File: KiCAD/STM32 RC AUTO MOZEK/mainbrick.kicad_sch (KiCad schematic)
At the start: 29 parts, among them J8 Conn_01x03_Socket, U10 ACS712xLCTR-20A, U11 ACS712xLCTR-20A, U13 STM32F030C8Tx, U2 SHT4x, U4 ACS712xLCTR-20A, U5 NRF24L01_Breakout, U7 ACS712xLCTR-20A, U8 ACS712xLCTR-20A, U9 ACS712xLCTR-20A, Y1 Crystal, Y2 Crystal

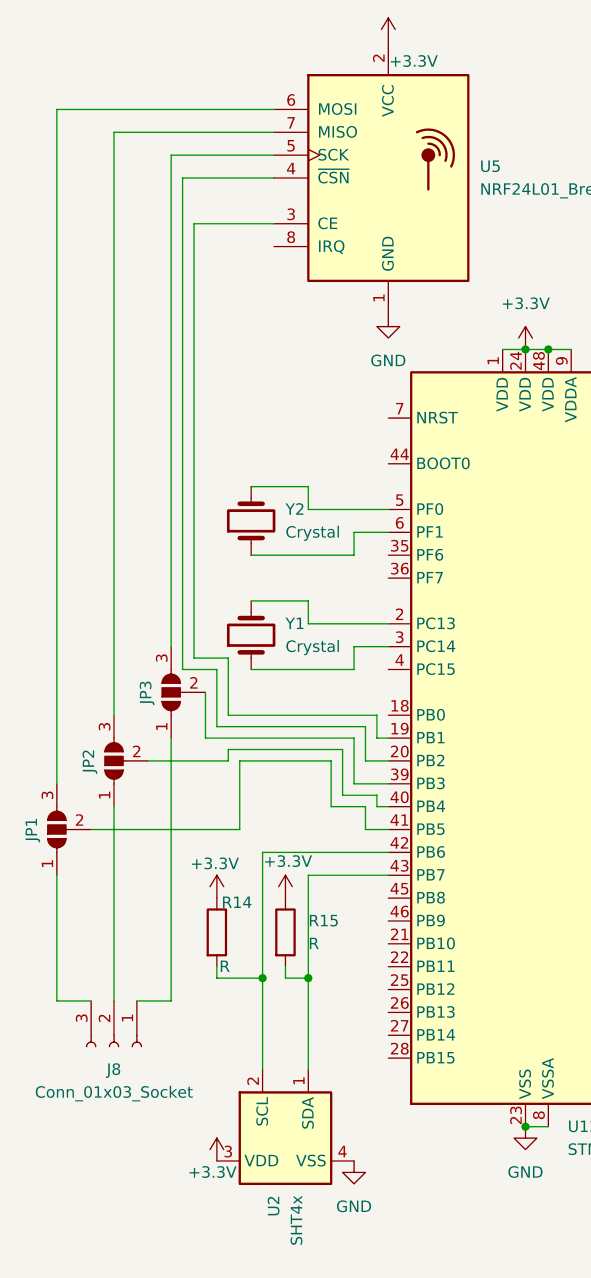
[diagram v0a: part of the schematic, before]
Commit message: i dont know
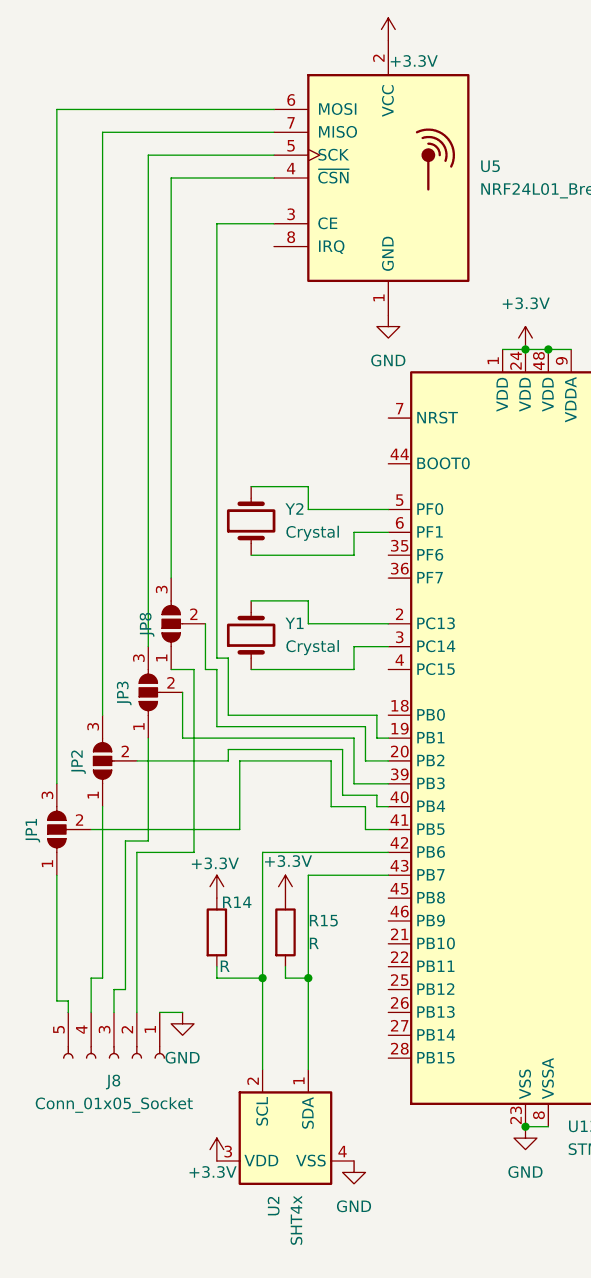
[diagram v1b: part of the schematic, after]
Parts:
- removed J8: Conn_01x03_Socket, Connector_Wire:SolderWire-0.5sqmm_1x03_P4.6mm_D0.9mm_OD2.1mm_Relief, symbol Connector:Conn_01x03_Socket
- added J8: Conn_01x05_Socket, Connector_Wire:SolderWire-0.5sqmm_1x05_P4.8mm_D0.9mm_OD2.3mm_Relief, symbol Connector:Conn_01x05_Socket
- added JP8: SolderJumper_3_Open, Jumper:SolderJumper-3_P1.3mm_Open_RoundedPad1.0x1.5mm_NumberLabels, symbol Jumper:SolderJumper_3_Open
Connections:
- net GND: now also J8.1 (Pin_1)
- net at U13.20 (PB2): now also JP8.2 (C); no longer U5.4 (~{CSN})
- net at JP3.1 (A): now also J8.3 (Pin_3)
- net at JP1.1 (A): now also J8.5 (Pin_5)
- net at JP2.1 (A): now also J8.4 (Pin_4)
- new net: J8.2 (Pin_2), JP8.1 (A)
- new net: JP8.3 (B), U5.4 (~{CSN})
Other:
- moved on the sheet: JP2, JP3
